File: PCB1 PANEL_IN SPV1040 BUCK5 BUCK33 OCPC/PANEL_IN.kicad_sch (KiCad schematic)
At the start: 0 parts

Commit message: EDITS N+1
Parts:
- added D12, D13, D14, D15, D16: D, symbol Device:D

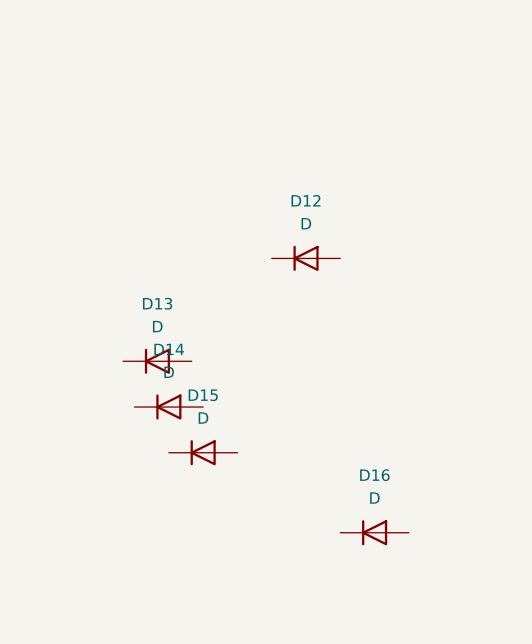
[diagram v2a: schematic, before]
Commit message: VCOMMIT
EDITS N+I
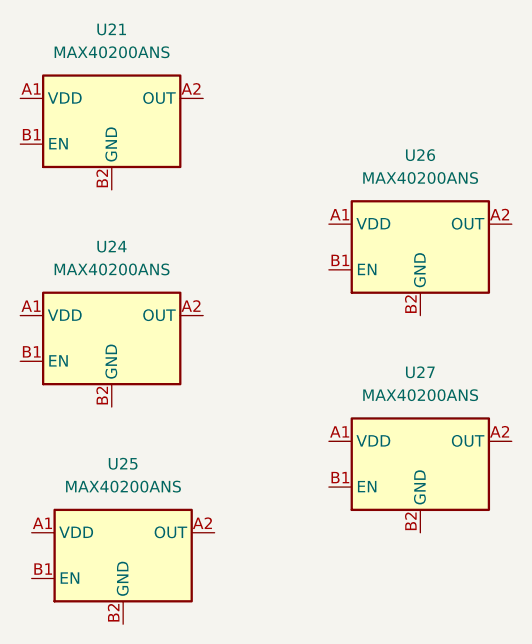
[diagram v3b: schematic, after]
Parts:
- removed D12, D13, D14, D15, D16: D, symbol Device:D
- added U21, U24, U25, U26, U27: MAX40200ANS, Package_TO_SOT_SMD:SOT-23-5, symbol Analog_Switch:MAX40200ANS
